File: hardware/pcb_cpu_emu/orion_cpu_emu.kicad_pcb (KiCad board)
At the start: 2 copper layers, 99.7 x 99.7 mm, 17 parts, among them J1 C96ABC, J2 GPIO 0, J3 GPIO 1, J4 SIGS, J5 SL0, J6 SL1

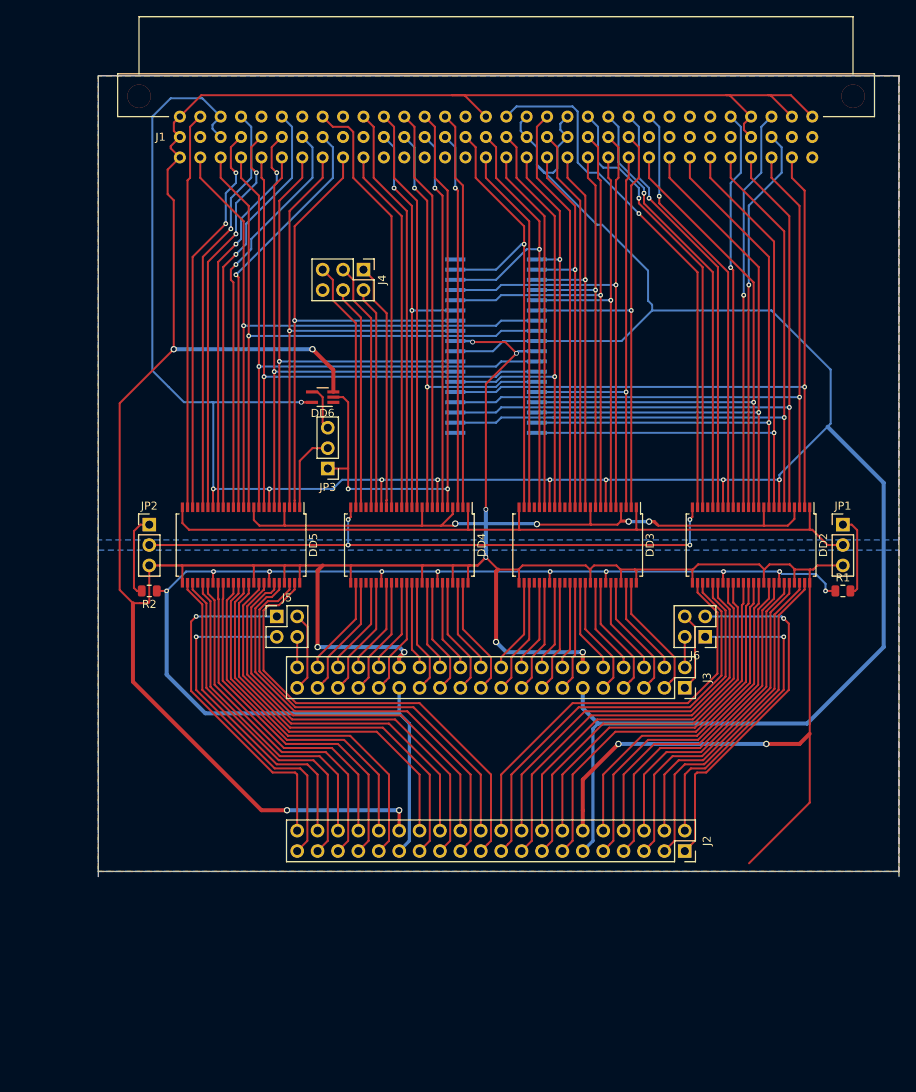
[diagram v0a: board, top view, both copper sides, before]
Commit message: Актуализированна аппаратная часть
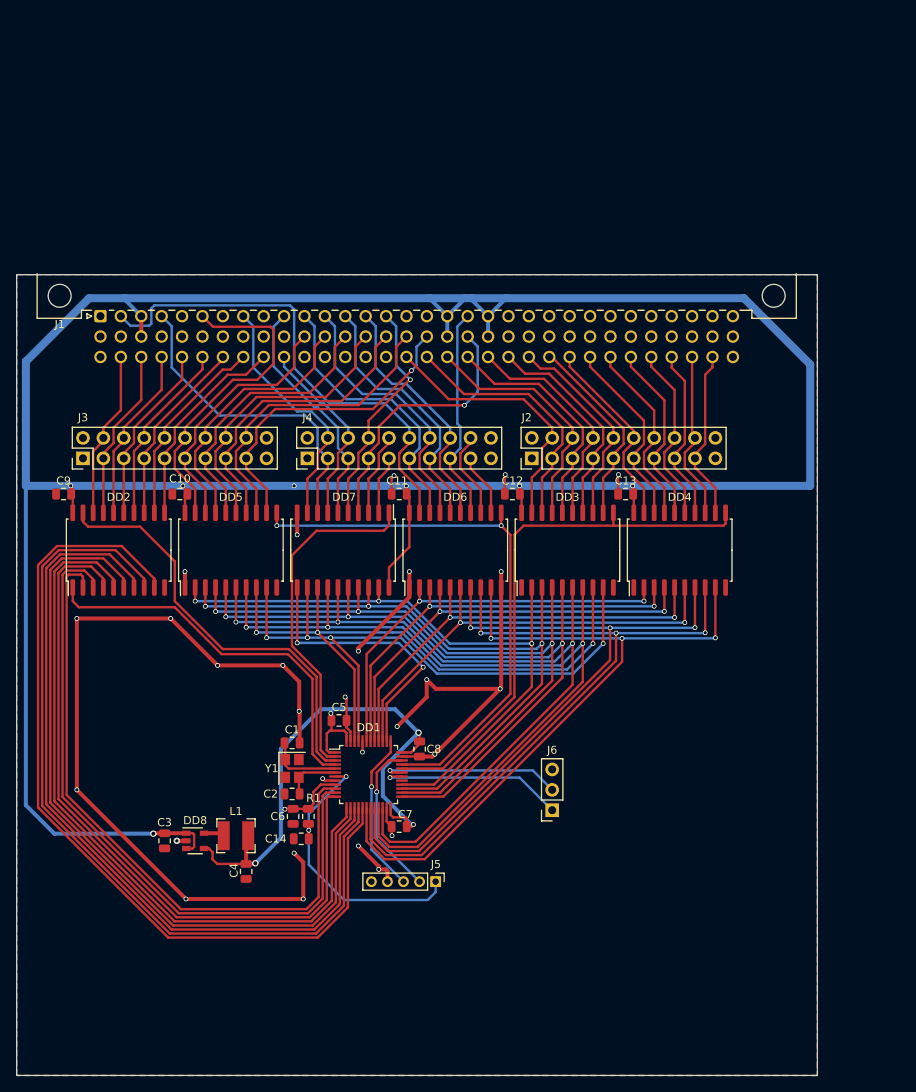
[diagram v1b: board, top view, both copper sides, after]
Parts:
- removed JP1: AB, Connector_PinHeader_2.54mm:PinHeader_1x03_P2.54mm_Vertical
- removed JP2: BA, Connector_PinHeader_2.54mm:PinHeader_1x03_P2.54mm_Vertical
- removed JP3: DB_DIR, Connector_PinHeader_2.54mm:PinHeader_1x03_P2.54mm_Vertical
- removed R2: 10k, Resistor_SMD:R_0805_2012Metric
- added C1: 22pf, Capacitor_SMD:C_0805_2012Metric, F.Cu at (94.0, 123.1)
- added C10: 100n, Capacitor_SMD:C_0805_2012Metric, F.Cu at (80.0, 92.1)
- added C11: 100n, Capacitor_SMD:C_0805_2012Metric, F.Cu at (107.3, 92.1)
- added C12: 100n, Capacitor_SMD:C_0805_2012Metric, F.Cu at (121.4, 92.1)
- added C13: 100n, Capacitor_SMD:C_0805_2012Metric, F.Cu at (135.5, 92.1)
- added C14: 4.7u, Capacitor_SMD:C_0805_2012Metric, F.Cu at (95.1, 135.0)
- added C2: 22pf, Capacitor_SMD:C_0805_2012Metric, F.Cu at (94.0, 129.4)
- added C3: 4.7u, Capacitor_SMD:C_0805_2012Metric, F.Cu at (78.1, 135.3)
- added C4: 4.7u, Capacitor_SMD:C_0805_2012Metric, F.Cu at (88.3, 139.1)
- added C5: 100n, Capacitor_SMD:C_0805_2012Metric, F.Cu at (99.8, 120.3)
- added C6: 100n, Capacitor_SMD:C_0805_2012Metric, F.Cu at (94.1, 132.2)
- added C7: 100n, Capacitor_SMD:C_0805_2012Metric, F.Cu at (107.3, 133.5)
- added C8: 100n, Capacitor_SMD:C_0805_2012Metric, F.Cu at (109.9, 123.8)
- added C9: 100n, Capacitor_SMD:C_0805_2012Metric, F.Cu at (65.5, 92.1)
- added DD7: IR33, Package_SO:SOIC-20W_7.5x12.8mm_P1.27mm, F.Cu at (100.3, 99.1)
- added DD8: LM3671MF, Package_TO_SOT_SMD:SOT-23-5, F.Cu at (81.9, 135.3)
- added L1: 4,7uH, Inductor_SMD:L_Bourns-SRN4018, F.Cu at (87.0, 134.6)
- added Y1: 8MHz, Crystal:Crystal_SMD_3225-4Pin_3.2x2.5mm, F.Cu at (94.0, 126.2)
- DD1: value CY7C1049B -> STM32F103CBTx; footprint Projects:SOJ-36 -> Package_QFP:LQFP-48_7x7mm_P0.5mm; moved to F.Cu
- DD2: value 74ALVC164245 -> AP6; footprint Package_SO:SSOP-48_7.5x15.9mm_P0.635mm -> Package_SO:SOIC-20W_7.5x12.8mm_P1.27mm
- DD3, DD4, DD5: value 74ALVC164245 -> IR33; footprint Package_SO:SSOP-48_7.5x15.9mm_P0.635mm -> Package_SO:SOIC-20W_7.5x12.8mm_P1.27mm
- DD6: value 74AHC1G04 -> IR33; footprint Package_TO_SOT_SMD:SOT-353_SC-70-5_Handsoldering -> Package_SO:SOIC-20W_7.5x12.8mm_P1.27mm
- J1: footprint orion:Socket_DIN41612-CaseC1-full-Male-96Pin-3rows -> Connector_DIN:DIN41612_C_3x32_Male_Horizontal_THT
- J2: value GPIO 0 -> Conn_02x10_Odd_Even; footprint Connector_PinSocket_2.54mm:PinSocket_2x20_P2.54mm_Vertical -> Connector_PinHeader_2.54mm:PinHeader_2x10_P2.54mm_Vertical
- J3: value GPIO 1 -> Conn_02x10_Odd_Even; footprint Connector_PinSocket_2.54mm:PinSocket_2x20_P2.54mm_Vertical -> Connector_PinHeader_2.54mm:PinHeader_2x10_P2.54mm_Vertical
- J4: value SIGS -> Conn_02x10_Odd_Even; footprint Connector_PinHeader_2.54mm:PinHeader_2x03_P2.54mm_Vertical -> Connector_PinHeader_2.54mm:PinHeader_2x10_P2.54mm_Vertical
- J5: value SL0 -> SWD; footprint Connector_PinHeader_2.54mm:PinHeader_2x02_P2.54mm_Vertical -> Connector_PinHeader_2.00mm:PinHeader_1x05_P2.00mm_Vertical
- J6: value SL1 -> UART; footprint Connector_PinHeader_2.54mm:PinHeader_2x02_P2.54mm_Vertical -> Connector_PinSocket_2.54mm:PinSocket_1x03_P2.54mm_Vertical
- R1: value 10k -> 1k
- moved J3 80.2 mm to (67.9, 87.6), turned to 90 degrees
- moved DD2 78.7 mm to (72.4, 99.1), turned to 90 degrees
- moved R1 72.2 mm to (96.0, 132.2), turned to -90 degrees
- moved J1 54.1 mm to (70.1, 69.9), turned to 0 degrees
- moved DD1 53.8 mm to (103.5, 127.0), turned to 0 degrees
- moved J2 52.5 mm to (123.8, 87.6), turned to 90 degrees
- moved J5 38.5 mm to (111.9, 140.3), turned to -90 degrees
- moved DD4 33.7 mm to (142.2, 99.1), turned to 90 degrees
- moved J6 28.8 mm to (126.4, 131.4)
- moved DD6 25.2 mm to (114.3, 99.1), turned to 90 degrees
- moved J4 24.5 mm to (95.9, 87.6), turned to 90 degrees
- moved DD5 1.42 mm to (86.4, 99.1), turned to 90 degrees
- moved DD3 1.42 mm to (128.3, 99.1), turned to 90 degrees
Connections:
- DD1 pad 1: /A13 -> +3V3
- DD1 pad 10: GND -> PA0
- DD1 pad 11: /D5 -> PA1
- DD1 pad 12: /D4 -> PA2
- DD1 pad 13: /~MWR -> PA3
- DD1 pad 14: /A8 -> PA4
- DD1 pad 15: /A7 -> PA5
- DD1 pad 16: /A6 -> PA6
- DD1 pad 17: /A5 -> PA7
- DD1 pad 18: /A4 -> PB0
- DD1 pad 19: (no net) -> PB1
- DD1 pad 2: /A12 -> OE2
- DD1 pad 20: /A3 -> PB2
- DD1 pad 21: /A2 -> PB10
- DD1 pad 22: /A1 -> PB11
- DD1 pad 23: /A0 -> GND
- DD1 pad 24: /MA14 -> +3V3
- DD1 pad 25: /D3 -> PB12
- DD1 pad 26: /D2 -> PB13
- DD1 pad 27: VCC -> PB14
- DD1 pad 28: GND -> PB15
- DD1 pad 29: /D1 -> (no net)
- DD1 pad 3: /A11 -> DOE
- DD1 pad 30: /D0 -> TX
- DD1 pad 31: /~MRD -> RX
- DD1 pad 32: /MA17 -> LE0
- DD1 pad 33: /MA18 -> LE1
- DD1 pad 34: /MA15 -> SWDIO
- DD1 pad 35: /MA16 -> GND
- DD1 pad 36: (no net) -> +3V3
- DD1 pad 4: /A10 -> DDIR
- DD1 pad 5: /A9 -> OSC_IN
- DD1 pad 6: /~CE0 -> OSC_OUT
- DD1 pad 7: /D7 -> NRST
- DD1 pad 8: /D6 -> GND
- DD1 pad 9: VCC -> +3V3
- DD2 pad 1: /AB -> DDIR
- DD2 pad 11: /A6 -> /D0
- DD2 pad 12: /A7 -> /D1
- DD2 pad 13: /INT50 -> /D2
- DD2 pad 14: /X0 -> /D3
- DD2 pad 15: (no net) -> /D4
- DD2 pad 16: /~IRQS -> /D5
- DD2 pad 17: /~IRQ4 -> /D6
- DD2 pad 18: VCC -> /D7
- DD2 pad 19: /~IRQ3 -> DOE
- DD2 pad 2: /A0 -> PA0
- DD2 pad 20: /~IRQ2 -> VCC
- DD2 pad 3: /A1 -> PA1
- DD2 pad 4: GND -> PA2
- DD2 pad 5: /A2 -> PA3
- DD2 pad 6: /A3 -> PA4
- DD2 pad 7: VCC -> PA5
- DD2 pad 8: /A4 -> PA6
- DD2 pad 9: /A5 -> PA7
- DD3 pad 1: /AB -> GND
- DD3 pad 11: /A11 -> LE0
- DD3 pad 12: /SND -> /A8
- DD3 pad 13: /A12 -> /A9
- DD3 pad 14: /~RFSH -> /A10
- DD3 pad 15: (no net) -> /A11
- DD3 pad 16: /A13 -> /A12
- DD3 pad 17: /MA14 -> /A13
- DD3 pad 18: VCC -> /A14
- DD3 pad 19: /A14 -> /A15
- DD3 pad 2: /~CE0 -> PB15
- DD3 pad 20: /MA15 -> VCC
- DD3 pad 3: /A8 -> PB14
- DD3 pad 4: GND -> PB13
- DD3 pad 5: /MA18 -> PB12
- DD3 pad 6: /A9 -> PB11
- DD3 pad 7: VCC -> PB10
- DD3 pad 8: /MA17 -> PB9
- DD3 pad 9: /A10 -> PB8
- DD4 pad 1: /AB -> GND
- DD4 pad 11: /~IORQ -> LE0
- DD4 pad 12: /~MRD -> /A0
- DD4 pad 13: /~BLIO -> /A1
- DD4 pad 14: /~WAIT -> /A2
- DD4 pad 15: (no net) -> /A3
- DD4 pad 16: /~BLRAM -> /A4
- DD4 pad 17: /S0 -> /A5
- DD4 pad 18: VCC -> /A6
- DD4 pad 19: /S1 -> /A7
- DD4 pad 2: /~RD -> PB7
- DD4 pad 20: /S2 -> VCC
- DD4 pad 3: /~UB -> PB6
- DD4 pad 4: GND -> PB5
- DD4 pad 5: /~WR -> PB4
- DD4 pad 6: /~VCE -> PB3
- DD4 pad 7: VCC -> PB2
- DD4 pad 8: /~MREQ -> PB1
- DD4 pad 9: /~MWR -> PB0
- DD5 pad 1: /DB -> GND
- DD5 pad 11: /D6 -> LE1
- DD5 pad 12: /D7 -> /MA14
- DD5 pad 13: /pFA -> /MA15
- DD5 pad 14: /pF8 -> /MA16
- DD5 pad 15: (no net) -> /MA17
- DD5 pad 16: /~M1 -> /MA18
- DD5 pad 17: /pFC -> /MA19
- DD5 pad 18: VCC -> /MA20
- DD5 pad 19: /~VO1 -> /M1
- DD5 pad 2: /D0 -> PB15
- DD5 pad 20: /~INTA -> VCC
- DD5 pad 3: /D1 -> PB14
- DD5 pad 4: GND -> PB13
- DD5 pad 5: /D2 -> PB12
- DD5 pad 6: /D3 -> PB11
- DD5 pad 7: VCC -> PB10
- DD5 pad 8: /D4 -> PB9
- DD5 pad 9: /D5 -> PB8
- DD6 pad 1: (no net) -> GND
- DD6 pad 2: /~WR -> PB7
- DD6 pad 3: GND -> PB6
- DD6 pad 4: Net-(DD6-Pad4) -> PB5
- DD6 pad 5: VCC -> PB4
- J2 pad 1: /P35 -> GND
- J2 pad 10: /P26 -> /A9
- J2 pad 11: VCC -> /A6
- J2 pad 12: GND -> /A7
- J2 pad 13: /P25 -> /A4
- J2 pad 14: /P24 -> /A5
- J2 pad 15: /P23 -> /A2
- J2 pad 16: /P22 -> /A3
- J2 pad 17: /P21 -> /A0
- J2 pad 18: /P20 -> /A1
- J2 pad 19: /P19 -> GND
- J2 pad 2: /P34 -> GND
- J2 pad 20: /P18 -> GND
- J2 pad 3: /P33 -> /A14
- J2 pad 4: /P32 -> /A15
- J2 pad 5: /P31 -> /A12
- J2 pad 6: /P30 -> /A13
- J2 pad 7: /P29 -> /A10
- J2 pad 8: /P28 -> /A11
- J2 pad 9: /P27 -> /A8
- J3 pad 1: /R35 -> GND
- J3 pad 10: /R26 -> /D1
- J3 pad 11: VCC -> /MA20
- J3 pad 12: GND -> /M1
- J3 pad 13: /R25 -> /MA18
- J3 pad 14: /R24 -> /MA19
- J3 pad 15: /R23 -> /MA16
- J3 pad 16: /R22 -> /MA17
- J3 pad 17: /R21 -> /MA14
- J3 pad 18: /R20 -> /MA15
- J3 pad 19: /R19 -> GND
- J3 pad 2: /R34 -> GND
- J3 pad 20: /R18 -> GND
- J3 pad 3: /R33 -> /D6
- J3 pad 4: /R32 -> /D7
- J3 pad 5: /R31 -> /D4
- J3 pad 6: /R30 -> /D5
- J3 pad 7: /R29 -> /D2
- J3 pad 8: /R28 -> /D3
- J3 pad 9: /R27 -> /D0
- J4 pad 1: /S0 -> GND
- J4 pad 2: /S1 -> GND
- J4 pad 3: /S2 -> /~INTA
- J4 pad 4: /S3 -> /~BLRAM
- J4 pad 5: /S4 -> /~BLIO
- J4 pad 6: Net-(J4-Pad6) -> /~WAIT
- J5 pad 1: /P0 -> NRST
- J5 pad 2: /R1 -> SWDIO
- J5 pad 3: /P1 -> SWCLK
- J5 pad 4: /R0 -> GND
- J6 pad 1: /P34 -> TX
- J6 pad 2: /R34 -> RX
- J6 pad 3: /P35 -> GND
- R1 pad 2: Net-(JP1-Pad1) -> NRST
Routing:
- net GND: track 611.4 -> 192.0 mm, vias 18 -> 28
- net PA7: track 0.00 -> 108.4 mm
- net PB10: track 0.00 -> 104.6 mm, vias 0 -> 3
- net PA6: track 0.00 -> 104.4 mm
- net PB11: track 0.00 -> 101.0 mm, vias 0 -> 3
- net PA5: track 0.00 -> 100.4 mm
- net /AB: track 96.6 -> 0.00 mm
- net PA4: track 0.00 -> 96.5 mm
- net PA3: track 0.00 -> 92.4 mm
- net PB0: track 0.00 -> 90.5 mm, vias 0 -> 3
- net PA2: track 0.00 -> 90.0 mm
- net PB12: track 0.00 -> 89.3 mm, vias 0 -> 3
- net PB1: track 0.00 -> 88.0 mm, vias 0 -> 3
- net PA1: track 0.00 -> 86.8 mm
- net PB13: track 0.00 -> 86.6 mm, vias 0 -> 3
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- added copper zone on B.Cu, net GND
- removed copper zone on B.Cu, net +3V3
- removed copper zone on B.Cu, net VCC
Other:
- outline, holes or cut-outs redrawn
- net class Default removed
